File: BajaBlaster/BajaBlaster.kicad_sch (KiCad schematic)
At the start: 0 parts

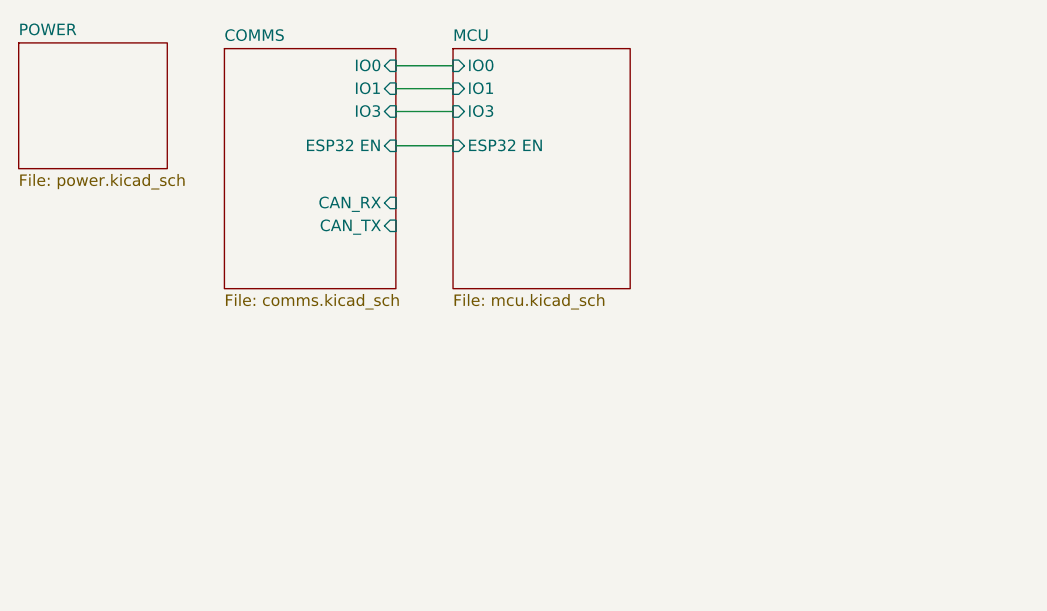
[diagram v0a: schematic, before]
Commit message: doing lots of small tweaks and fixups
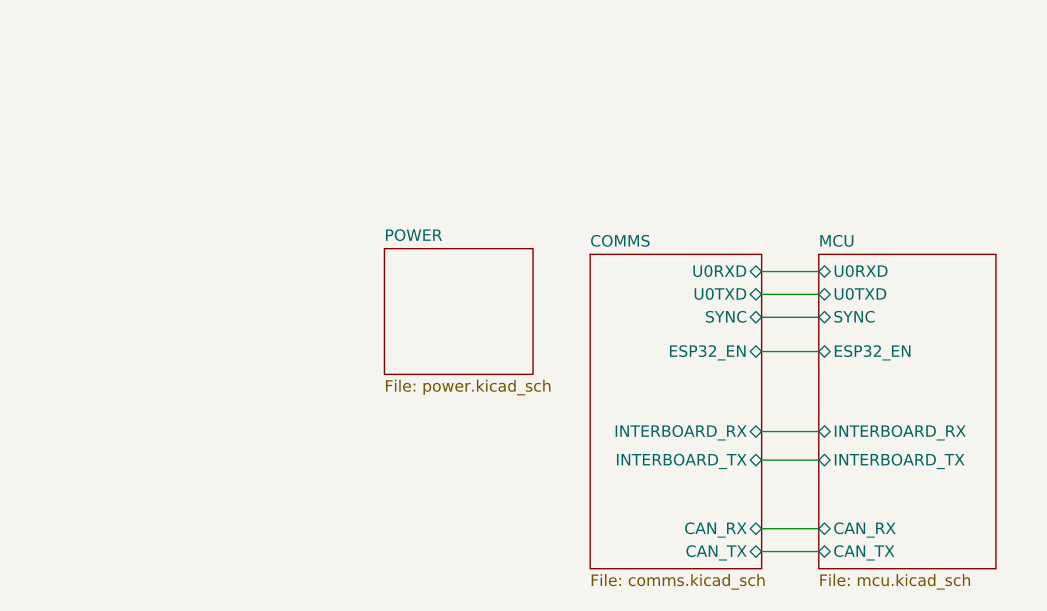
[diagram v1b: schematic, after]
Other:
- sheet COMMS ports: added ESP32_EN, INTERBOARD_RX, INTERBOARD_TX, SYNC, U0RXD, U0TXD; removed ESP32 EN, IO0, IO1, IO3
- sheet MCU ports: added CAN_RX, CAN_TX, ESP32_EN, INTERBOARD_RX, INTERBOARD_TX, SYNC, U0RXD, U0TXD; removed ESP32 EN, IO0, IO1, IO3
- title: (none) -> BAJA_BLASTER_REV_A
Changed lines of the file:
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@@
 	(generator_version "10.0")
 	(paper "A5")
-	(wire
-		(pts
-			(xy 58.42 25.4) (xy 64.77 25.4)
-		)
-		(stroke
-			(width 0)
-			(type default)
-		)
-	)
-	(wire
-		(pts
-			(xy 58.42 29.21) (xy 64.77 29.21)
-		)
-		(stroke
-			(width 0)
-			(type default)
-		)
-	)
-	(wire
-		(pts
-			(xy 58.42 20.32) (xy 64.77 20.32)
-		)
-		(stroke
-			(width 0)
-			(type default)
-		)
-	)
-	(wire
-		(pts
-			(xy 58.42 22.86) (xy 64.77 22.86)
+	(title_block
+		(title "BAJA_BLASTER_REV_A")
+	)
+	(wire
+		(pts
+			(xy 99.06 60.96) (xy 105.41 60.96)
+		)
+		(stroke
+			(width 0)
+			(type default)
+		)
+	)
+	(wire
+		(pts
+			(xy 99.06 71.755) (xy 105.41 71.755)
+		)
+		(stroke
+			(width 0)
+			(type default)
+		)
+	)
+	(wire
+		(pts
+			(xy 99.06 48.26) (xy 105.41 48.26)
+		)
+		(stroke
+			(width 0)
+			(type default)
+		)
+	)
+	(wire
+		(pts
+			(xy 99.06 64.135) (xy 105.41 64.135)
+		)
+		(stroke
+			(width 0)
+			(type default)
+		)
+	)
+	(wire
+		(pts
+			(xy 99.06 74.295) (xy 105.41 74.295)
+		)
+		(stroke
+			(width 0)
+			(type default)
+		)
+	)
+	(wire
+		(pts
+			(xy 99.06 52.07) (xy 105.41 52.07)
+		)
+		(stroke
+			(width 0)
+			(type default)
+		)
+	)
+	(wire
+		(pts
+			(xy 99.06 43.18) (xy 105.41 43.18)
+		)
+		(stroke
+			(width 0)
+			(type default)
+		)
+	)
+	(wire
+		(pts
+			(xy 99.06 45.72) (xy 105.41 45.72)
 		)
 		(stroke
@@
 	)
 	(sheet
-		(at 39.37 18.415)
-		(size 19.05 26.67)
+		(at 80.01 41.275)
+		(size 19.05 34.925)
 		(exclude_from_sim no)
 		(in_bom yes)
@@
 		)
 		(property "Sheetname" "COMMS"
-			(at 39.37 17.7034 0)
+			(at 80.01 40.5634 0)
 			(show_name no)
 			(do_not_autoplace no)
@@
 		)
 		(property "Sheetfile" "comms.kicad_sch"
-			(at 39.37 45.6696 0)
+			(at 80.01 76.7846 0)
 			(show_name no)
 			(do_not_autoplace no)
@@
 			)
 		)
-		(pin "IO1" input
-			(at 58.42 22.86 0)
-			(effects
-				(font
-					(size 1.27 1.27)
-				)
-				(justify right)
-			)
-		)
-		(pin "IO3" input
-			(at 58.42 25.4 0)
-			(effects
-				(font
-					(size 1.27 1.27)
-				)
-				(justify right)
-			)
-		)
-		(pin "ESP32 EN" input
-			(at 58.42 29.21 0)
-			(effects
-				(font
-					(size 1.27 1.27)
-				)
-				(justify right)
-			)
-		)
-		(pin "IO0" input
-			(at 58.42 20.32 0)
-			(effects
-				(font
-					(size 1.27 1.27)
-				)
-				(justify right)
-			)
-		)
-		(pin "CAN_TX" input
-			(at 58.42 38.1 0)
-			(effects
-				(font
-					(size 1.27 1.27)
-				)
-				(justify right)
-			)
-		)
-		(pin "CAN_RX" input
-			(at 58.42 35.56 0)
+		(pin "ESP32_EN" bidirectional
+			(at 99.06 52.07 0)
+			(effects
+				(font
+					(size 1.27 1.27)
+				)
+				(justify right)
+			)
+		)
+		(pin "CAN_TX" bidirectional
+			(at 99.06 74.295 0)
+			(effects
+				(font
+					(size 1.27 1.27)
+				)
+				(justify right)
+			)
+		)
+		(pin "CAN_RX" bidirectional
+			(at 99.06 71.755 0)
+			(effects
+				(font
+					(size 1.27 1.27)
+				)
+				(justify right)
+			)
+		)
+		(pin "U0RXD" bidirectional
+			(at 99.06 43.18 0)
+			(effects
+				(font
+					(size 1.27 1.27)
+				)
+				(justify right)
+			)
+		)
+		(pin "INTERBOARD_RX" bidirectional
+			(at 99.06 60.96 0)
+			(effects
+				(font
+					(size 1.27 1.27)
+				)
+				(justify right)
+			)
+		)
+		(pin "INTERBOARD_TX" bidirectional
+			(at 99.06 64.135 0)
+			(effects
+				(font
+					(size 1.27 1.27)
+				)
+				(justify right)
+			)
+		)
+		(pin "U0TXD" bidirectional
+			(at 99.06 45.72 0)
+			(effects
+				(font
+					(size 1.27 1.27)
+				)
+				(justify right)
+			)
+		)
+		(pin "SYNC" bidirectional
+			(at 99.06 48.26 0)
 			(effects
 				(font
@@
 	)
 	(sheet
-		(at 16.51 17.78)
+		(at 57.15 40.64)
 		(size 16.51 13.97)
 		(exclude_from_sim no)
@@
 		)
 		(property "Sheetname" "POWER"
-			(at 16.51 17.0684 0)
+			(at 57.15 39.9284 0)
 			(show_name no)
 			(do_not_autoplace no)
@@
 		)
 		(property "Sheetfile" "power.kicad_sch"
-			(at 16.51 32.3346 0)
+			(at 57.15 55.1946 0)
 			(show_name no)
 			(do_not_autoplace no)
@@
 	)
 	(sheet
-		(at 64.77 18.415)
-		(size 19.685 26.67)
+		(at 105.41 41.275)
+		(size 19.685 34.925)
 		(exclude_from_sim no)
 		(in_bom yes)
@@
 		)
 		(property "Sheetname" "MCU"
-			(at 64.77 17.7034 0)
+			(at 105.41 40.5634 0)
 			(show_name no)
 			(do_not_autoplace no)
@@
 		)
 		(property "Sheetfile" "mcu.kicad_sch"
-			(at 64.77 45.6696 0)
+			(at 105.41 76.7846 0)
 			(show_name no)
 			(do_not_autoplace no)
@@
 			)
 		)
-		(pin "IO1" input
-			(at 64.77 22.86 180)
-			(effects
-				(font
-					(size 1.27 1.27)
-				)
-				(justify left)
-			)
-		)
-		(pin "IO3" input
-			(at 64.77 25.4 180)
-			(effects
-				(font
-					(size 1.27 1.27)
-				)
-				(justify left)
-			)
-		)
-		(pin "IO0" input
-			(at 64.77 20.32 180)
-			(effects
-				(font
-					(size 1.27 1.27)
-				)
-				(justify left)
-			)
-		)
-		(pin "ESP32 EN" input
-			(at 64.77 29.21 180)
-			(effects
-				(font
+		(pin "ESP32_EN" bidirectional
+			(at 105.41 52.07 180)
+			(effects
+				(font
+					(size 1.27 1.27)
+				)
+				(justify left)
+			)
+		)
+		(pin "U0TXD" bidirectional
+			(at 105.41 45.72 180)
+			(effects
+				(font
+					(size 1.27 1.27)
+				)
+				(justify left)
+			)
+		)
+		(pin "U0RXD" bidirectional
+			(at 105.41 43.18 180)
+			(effects
+				(font
+					(size 1.27 1.27)
+				)
+				(justify left)
+			)
+		)
+		(pin "INTERBOARD_RX" bidirectional
+			(at 105.41 60.96 180)
+			(effects
+				(font
+					(size 1.27 1.27)
+				)
+				(justify left)
+			)
+		)
+		(pin "INTERBOARD_TX" bidirectional
+			(at 105.41 64.135 180)
+			(effects
+				(font
+					(size 1.27 1.27)
+				)
+				(justify left)
+			)
+		)
+		(pin "CAN_RX" bidirectional
+			(at 105.41 71.755 180)
+			(effects
+				(font
+					(size 1.27 1.27)
+				)
+				(justify left)
+			)
+		)
+		(pin "CAN_TX" bidirectional
+			(at 105.41 74.295 180)
+			(effects
+				(font
+					(size 1.27 1.27)
+				)
+				(justify left)
+			)
+		)
+		(pin "SYNC" bidirectional
+			(at 105.41 48.26 180)
+			(effects
+				(font
